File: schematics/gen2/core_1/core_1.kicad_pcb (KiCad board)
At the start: 2 copper layers, 84.3 x 8.4 mm, 10 parts, among them U1 74LS00, U2 74LS04, U3 74LS109, U4 74LS02

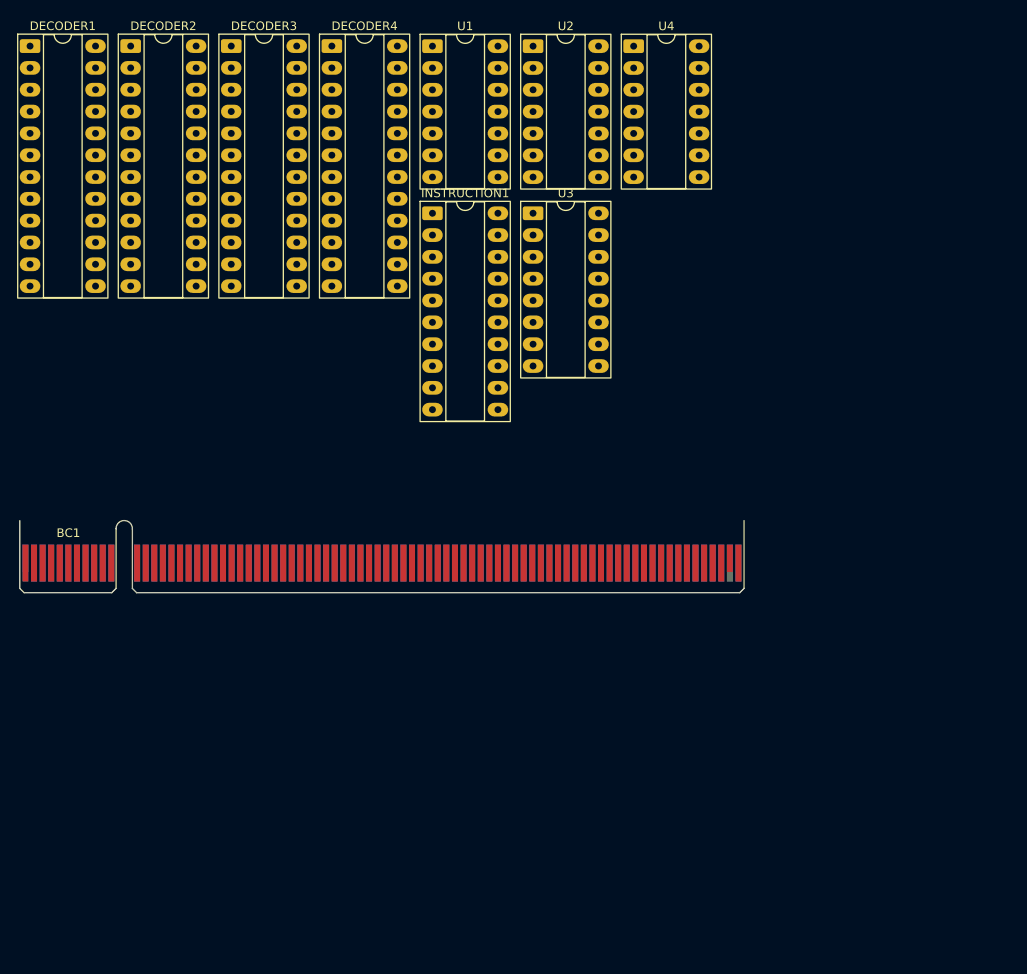
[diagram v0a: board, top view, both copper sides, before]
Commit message: core1 completed
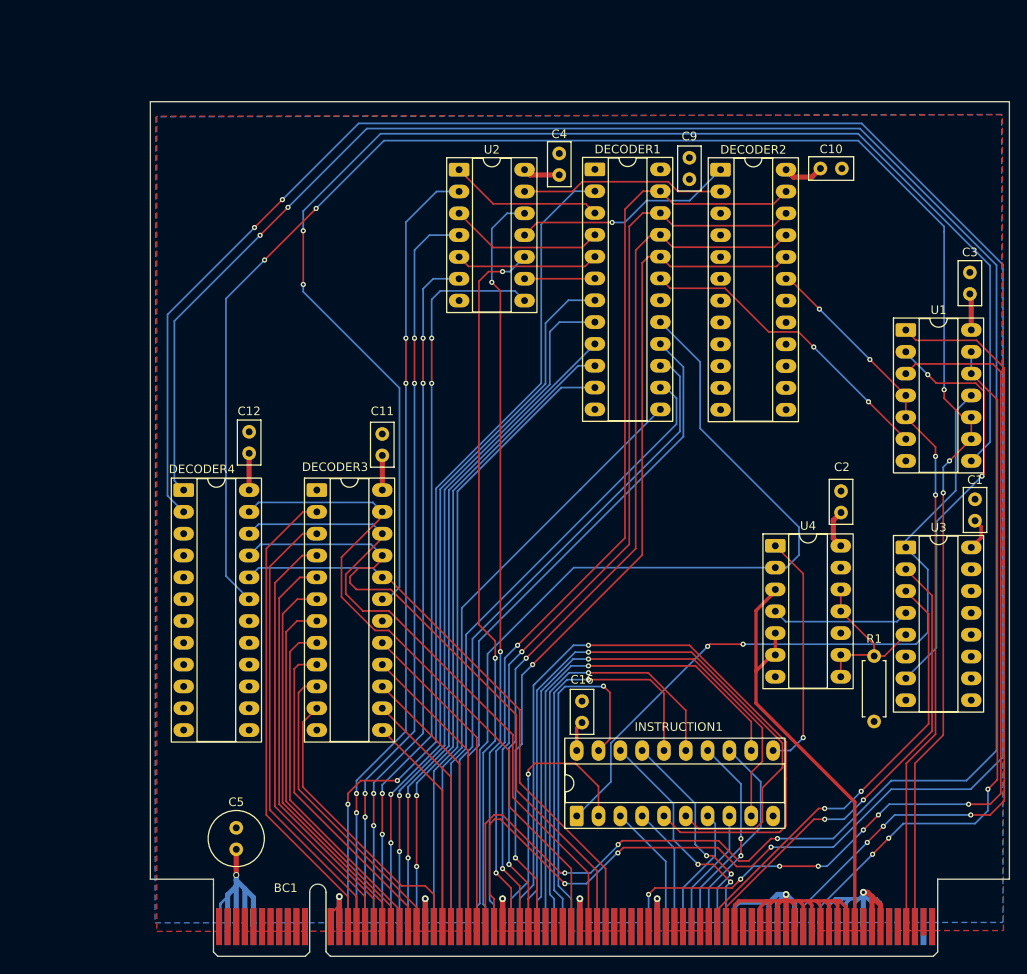
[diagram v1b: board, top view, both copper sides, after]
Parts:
- added C1: C, Capacitor_THT:C_Disc_D5.0mm_W2.5mm_P2.50mm, F.Cu at (191.0, 79.2)
- added C10: C, Capacitor_THT:C_Disc_D5.0mm_W2.5mm_P2.50mm, F.Cu at (173.0, 38.2)
- added C11: C, Capacitor_THT:C_Disc_D5.0mm_W2.5mm_P2.50mm, F.Cu at (122.0, 71.7)
- added C12: C, Capacitor_THT:C_Disc_D5.0mm_W2.5mm_P2.50mm, F.Cu at (106.5, 71.4)
- added C16: C, Capacitor_THT:C_Disc_D5.0mm_W2.5mm_P2.50mm, F.Cu at (145.2, 102.8)
- added C2: C, Capacitor_THT:C_Disc_D5.0mm_W2.5mm_P2.50mm, F.Cu at (175.4, 78.3)
- added C3: C, Capacitor_THT:C_Disc_D5.0mm_W2.5mm_P2.50mm, F.Cu at (190.4, 52.9)
- added C4: C, Capacitor_THT:C_Disc_D5.0mm_W2.5mm_P2.50mm, F.Cu at (142.6, 39.0)
- added C5: C, Capacitor_THT:C_Radial_D6.3mm_H5.0mm_P2.50mm, F.Cu at (105.0, 117.5)
- added C9: C, Capacitor_THT:C_Disc_D5.0mm_W2.5mm_P2.50mm, F.Cu at (157.8, 39.5)
- added R1: 5kOhm, Resistor_THT:R_Axial_DIN0207_L6.3mm_D2.5mm_P7.62mm_Horizontal, F.Cu at (179.2, 102.6)
- moved INSTRUCTION1 72.1 mm to (144.6, 113.6), turned to 90 degrees
- moved DECODER2 70.2 mm to (161.4, 38.4)
- moved DECODER1 67.3 mm to (146.8, 38.4)
- moved U1 64.2 mm to (182.9, 57.0)
- moved U4 60.5 mm to (167.8, 82.2)
- moved U3 58.3 mm to (182.9, 82.4)
- moved DECODER4 54.5 mm to (98.9, 75.7)
- moved DECODER3 52.6 mm to (114.4, 75.7)
- moved BC1 47.9 mm to (103.0, 126.5)
- moved U2 16.8 mm to (130.9, 38.4)
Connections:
- U4 pad 11: Net-(R2-Pad2) -> Net-(U3A-~{S})
- U4 pad 12: Net-(R2-Pad2) -> Net-(U3A-~{S})
- U4 pad 8: Net-(R2-Pad2) -> Net-(U3A-~{S})
- U4 pad 9: Net-(R2-Pad2) -> Net-(U3A-~{S})
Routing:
- net /~{IntAck}: track 0.00 -> 277.5 mm, vias 0 -> 5
- net /~{ALUWriter}: track 0.00 -> 270.8 mm, vias 0 -> 5
- net /R4: track 0.00 -> 217.5 mm, vias 0 -> 5
- net Net-(DECODER3-E1): track 0.00 -> 164.7 mm, vias 0 -> 2
- net GND: track 0.00 -> 151.6 mm, vias 0 -> 7
- net /L0: track 0.00 -> 111.3 mm, vias 0 -> 2
- net Net-(BC1-STATE15): track 0.00 -> 110.6 mm, vias 0 -> 7
- net /L1: track 0.00 -> 108.5 mm, vias 0 -> 2
- net /~{InstructionReader}: track 0.00 -> 107.1 mm
- net /L2: track 0.00 -> 105.2 mm, vias 0 -> 2
- net /L3: track 0.00 -> 102.4 mm, vias 0 -> 2
- net /~{MemoryReader}: track 0.00 -> 101.4 mm, vias 0 -> 2
- net /IRQ: track 0.00 -> 94.5 mm, vias 0 -> 3
- net /SPHighReader: track 0.00 -> 92.1 mm, vias 0 -> 4
- net /STATE1: track 0.00 -> 89.8 mm, vias 0 -> 1
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- added copper zone on B.Cu, net GND
- added copper zone on F.Cu, net VCC
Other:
- board size 84.3 x 8.4 mm -> 100 x 91.1 mm
